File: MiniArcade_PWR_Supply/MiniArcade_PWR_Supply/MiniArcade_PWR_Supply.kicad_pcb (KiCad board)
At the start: 2 copper layers, 60 x 55 mm, 17 parts, among them IC1 MIC94310-SYM5-TR, J1 Conn_01x03, J2 Conn_01x02_Pin, J3 Conn_01x02_Pin, U1 2479

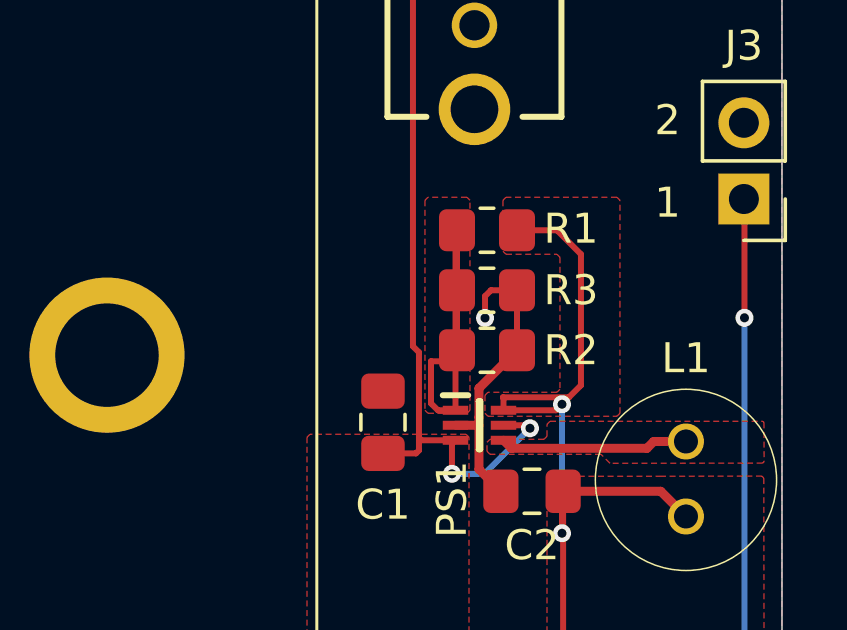
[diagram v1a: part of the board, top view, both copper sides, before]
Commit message: 08 12 2025
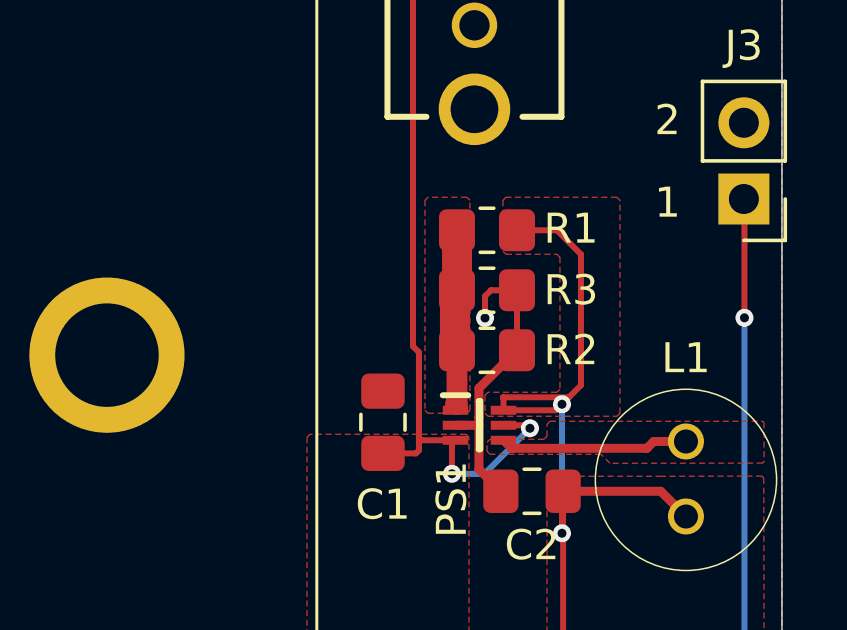
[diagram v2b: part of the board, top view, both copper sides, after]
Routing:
- net Net-(PS1-FB): track 13.4 -> 6.05 mm
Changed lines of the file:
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@@
+	)
+	(segment
+		(start 149.167926 127.582074)
+		(end 149.167926 129.381074)
+		(width 0.7)
+		(layer "F.Cu")
+		(net 12)
 	)
 	(segment
@@
 	)
 	(segment
-		(start 149.167926 125.582074)
-		(end 149.167926 123.582074)
-		(width 0.2)
+		(start 149.1 127.514148)
+		(end 149.1 125.65)
+		(width 1)
 		(layer "F.Cu")
 		(net 12)
 	)
 	(segment
-		(start 148.301 129.351)
-		(end 148.301 127.95)
-		(width 0.2)
-		(layer "F.Cu")
-		(net 12)
-	)
-	(segment
-		(start 148.8 127.95)
-		(end 149.167926 127.582074)
-		(width 0.2)
-		(layer "F.Cu")
-		(net 12)
-	)
-	(segment
-		(start 148.532074 129.582074)
-		(end 148.301 129.351)
-		(width 0.2)
-		(layer "F.Cu")
-		(net 12)
-	)
-	(segment
-		(start 148.301 127.95)
-		(end 148.8 127.95)
-		(width 0.2)
-		(layer "F.Cu")
-		(net 12)
-	)
-	(segment
-		(start 149.117926 129.582074)
-		(end 149.117926 123.632074)
+		(start 149.167926 129.532074)
+		(end 149.117926 129.582074)
 		(width 0.2)
 		(layer "F.Cu")
@@
 	(segment
 		(start 149.167926 127.582074)
-		(end 149.167926 125.582074)
-		(width 0.2)
+		(end 149.1 127.514148)
+		(width 1)
 		(layer "F.Cu")
 		(net 12)
 	)
 	(segment
-		(start 149.117926 129.582074)
-		(end 148.532074 129.582074)
-		(width 0.2)
+		(start 149.167926 125.582074)
+		(end 149.167926 123.582074)
+		(width 1)
+		(layer "F.Cu")
+		(net 12)
+	)
+	(segment
+		(start 149.167926 129.381074)
+		(end 149.117926 129.381074)
+		(width 0.7)
+		(layer "F.Cu")
+		(net 12)
+	)
+	(segment
+		(start 149.1 125.65)
+		(end 149.167926 125.582074)
+		(width 1)
 		(layer "F.Cu")
 		(net 12)
@@
 			(thermal_gap 0.5)
 			(thermal_bridge_width 0.5)
-			(island_removal_mode 1)
-			(island_area_min 9.999999)
 		)
 		(polygon
